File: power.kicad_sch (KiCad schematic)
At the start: 80 parts, among them CON2 BARREL_JACK, P5 CONN_01X01, P7 CONN_01X01, P8 CONN_01X01, U17 LMR51420, U18 LMR51420, U19 LMR51420, U20 LP5907-3.0, U21 LP2985A-10DBVR, U22 LD3920, U23 LD3920, U24 LD3920, U25 BU33SD5WG

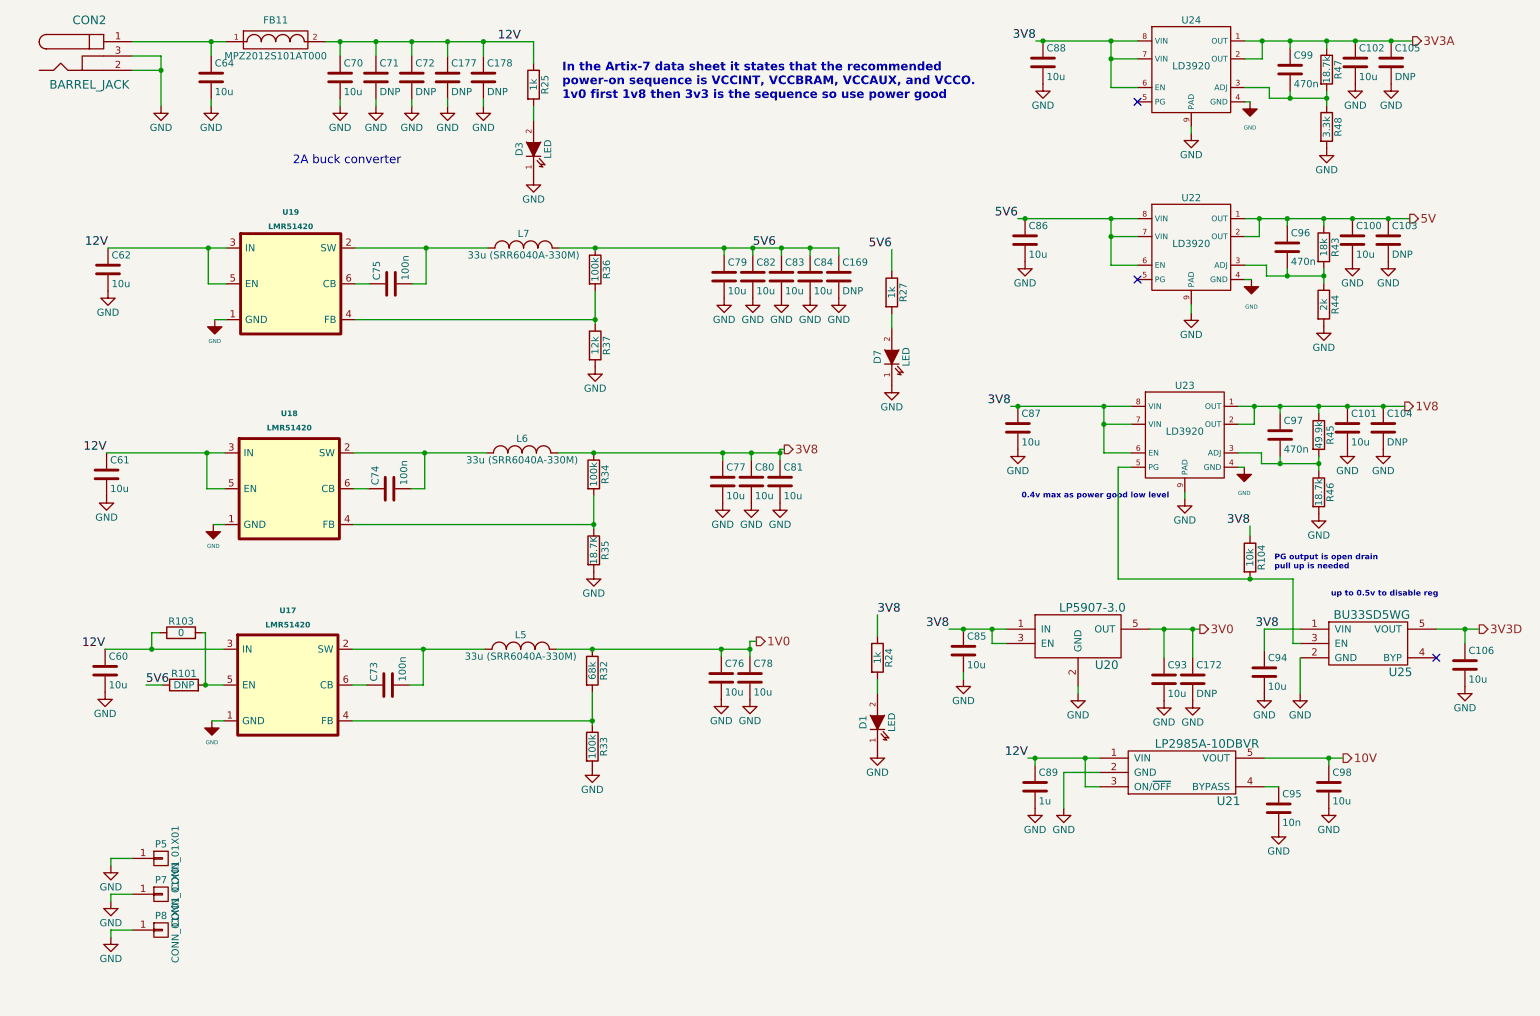
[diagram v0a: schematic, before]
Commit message: checks are done.
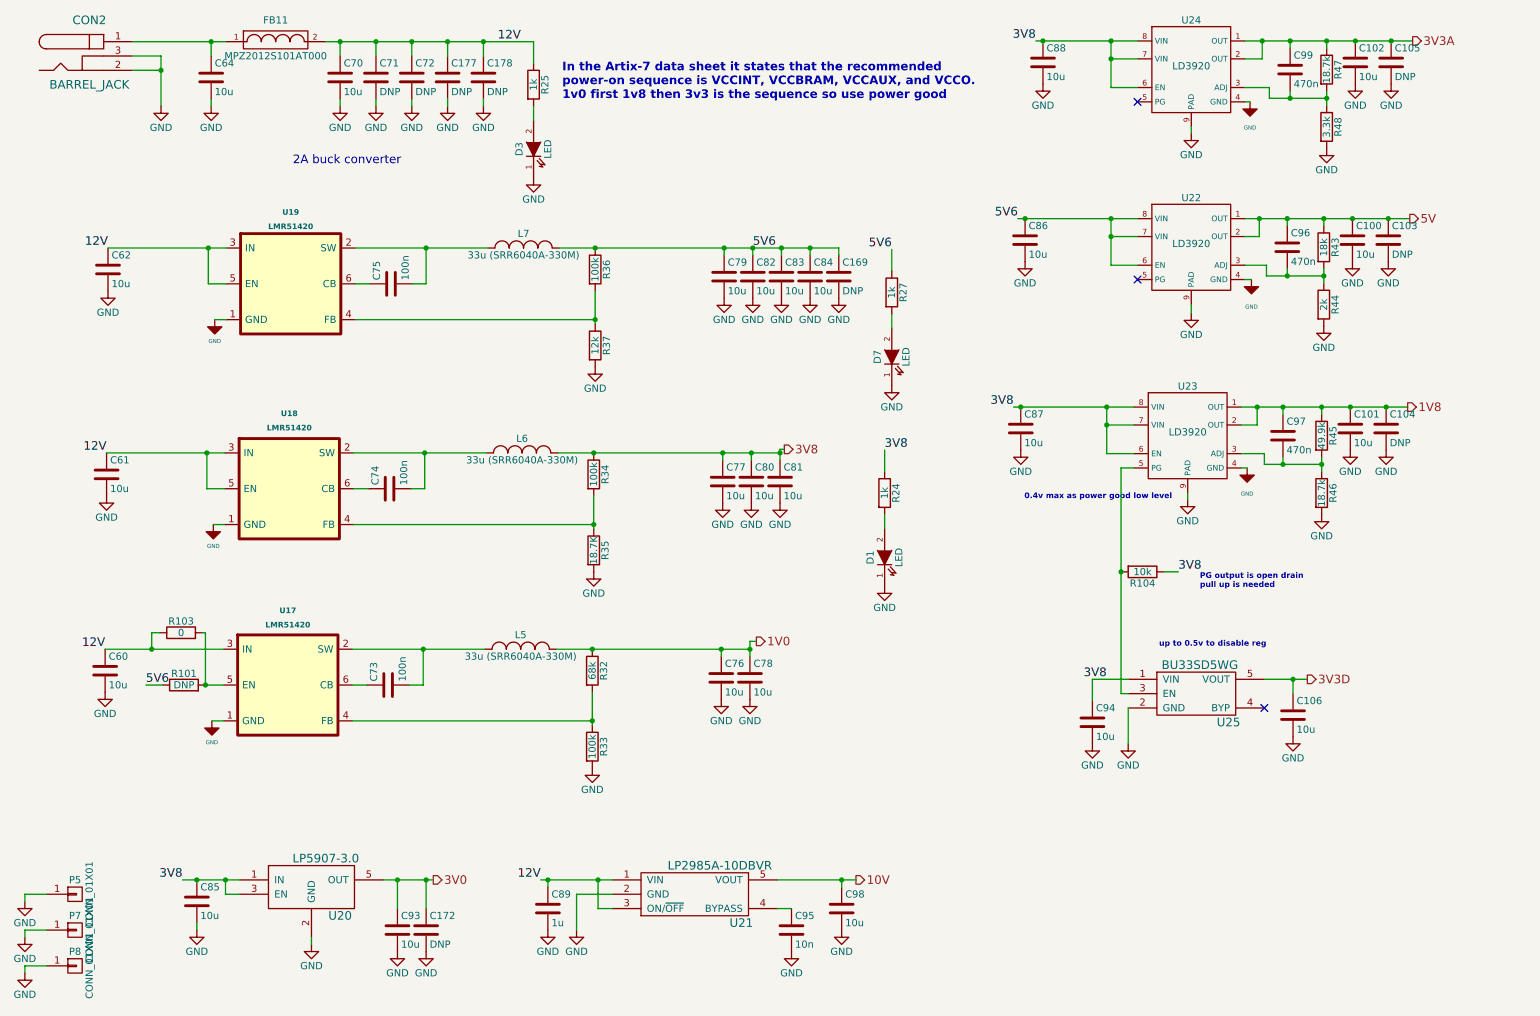
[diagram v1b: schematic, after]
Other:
- moved on the sheet: C101, C104, C106, C172, C85, C87, C89, C93, C94, C95, C97, C98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
